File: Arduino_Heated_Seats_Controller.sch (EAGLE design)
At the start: 13 parts, among them U1 ULN2003AN, U2 M54564P

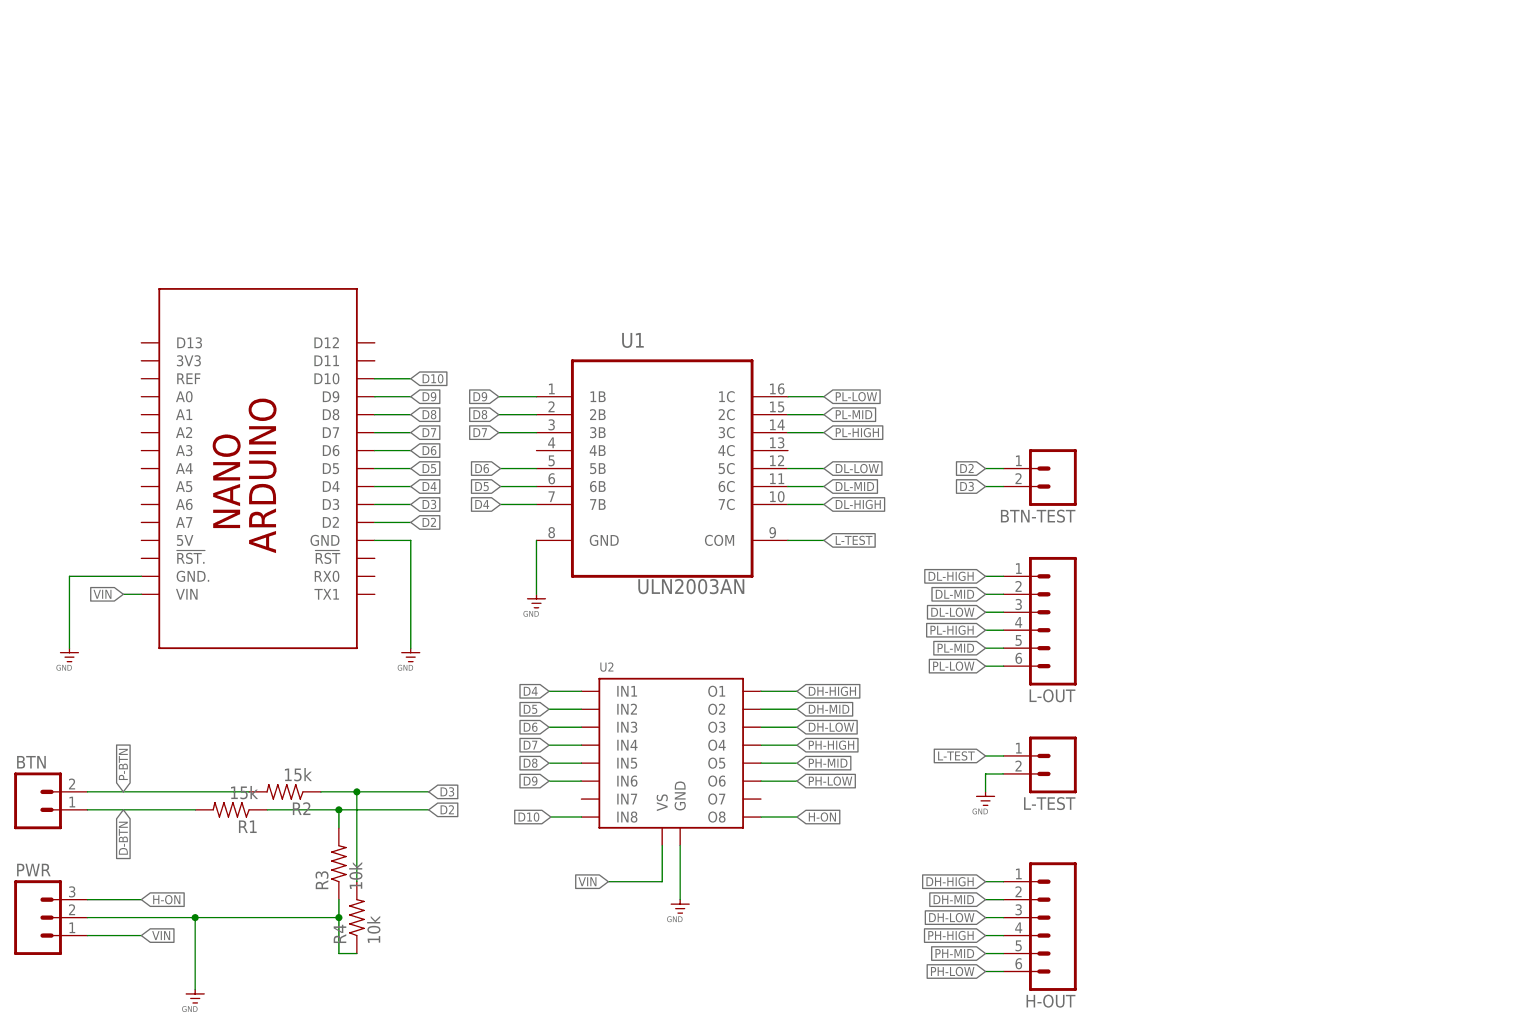
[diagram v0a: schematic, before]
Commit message: Initial work on rev3 underway (time for some sleep).
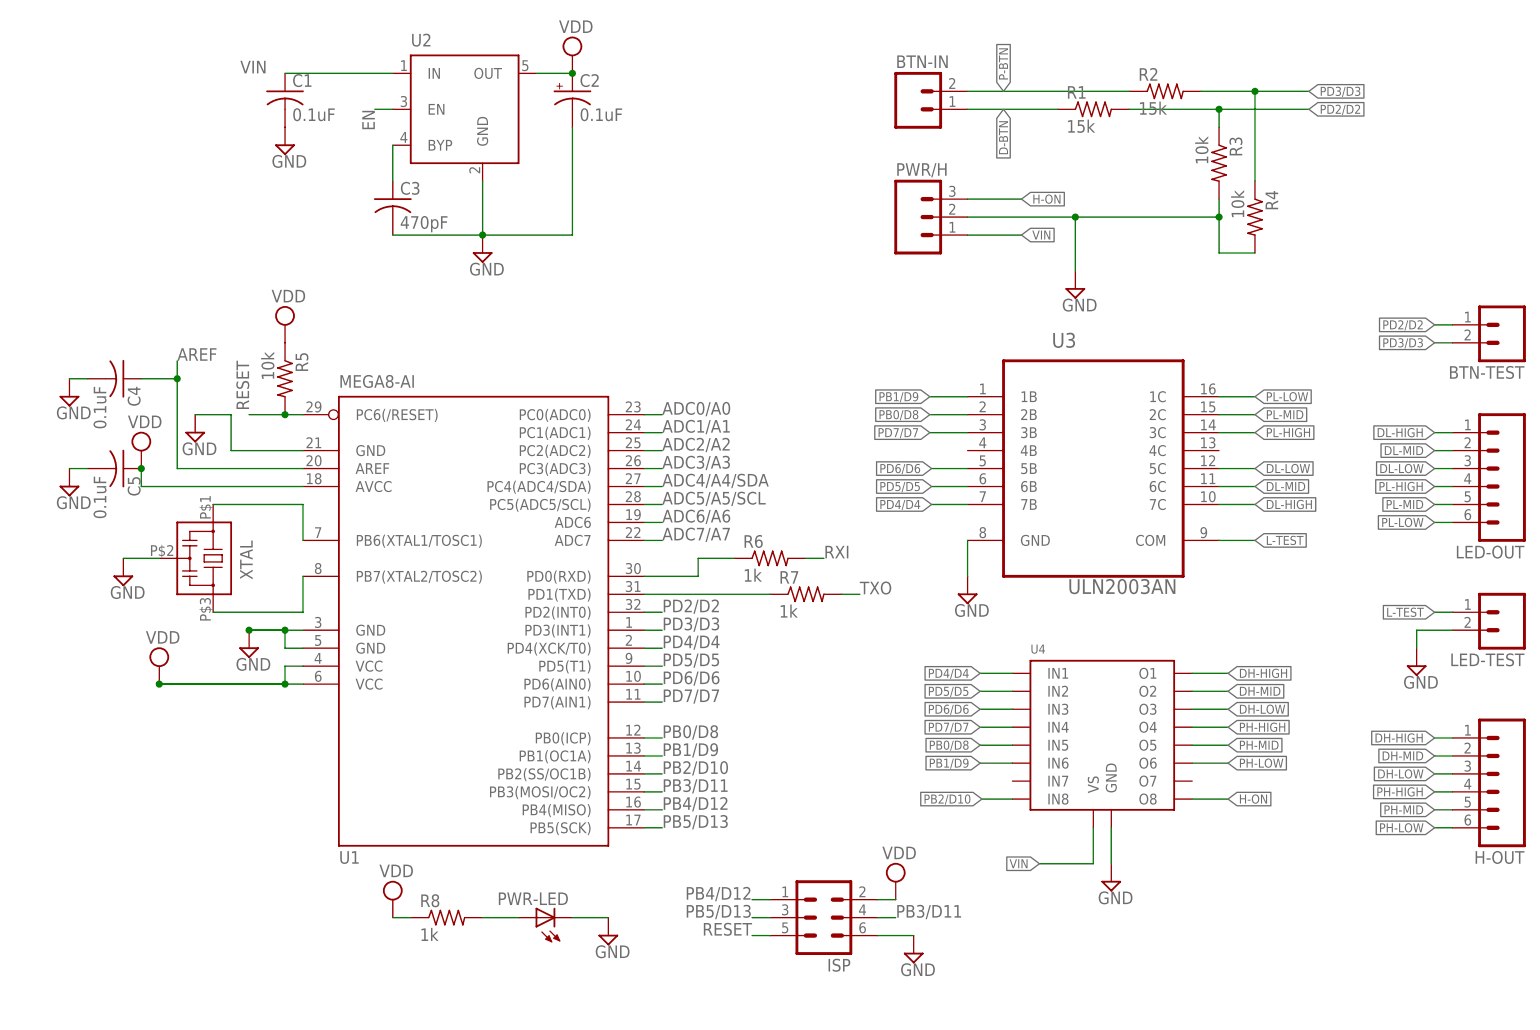
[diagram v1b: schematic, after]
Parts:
- removed BTN, L-TEST: M02PTH, SparkFun-Connectors:M02PTH
- removed L-OUT: (no value), SparkFun-Connectors:M06SIP
- removed PCB1: ARDUINO_NANO, E14_Arduino:ARDUINO_NANO
- removed PWR: (no value), SparkFun-Connectors:M03PTH
- added BTN-IN, LED-TEST: M02PTH, SparkFun-Connectors:M02PTH
- added C1, C4, C5: 0.1uF, rcl:C-USC0603
- added C2: 0.1uF, rcl:CPOL-USCT3216
- added C3: 470pF, rcl:C-USC0603
- added ISP: (no value), con-lstb:MA03-2
- added LED-OUT: (no value), SparkFun-Connectors:M06SIP
- added PWR-LED: (no value), led:LEDCHIP-LED0603
- added PWR/H: (no value), SparkFun-Connectors:M03PTH
- added R5: 10k, resistor:R-US_R0603
- added R6, R7, R8: 1k, resistor:R-US_R0603
- added U3: ULN2003AN, Texas Instruments_By_element14_Batch_1:ULN2003ANE4
- added U4: M54564FP, M54564P-FP:M54564FP
- added XTAL: CSTCE_V, murata-filter:CSTCE_V
- R1, R2, R3, R4: device SparkFun-Resistors:RESISTOR0603-RES -> resistor:R-US_R0603
- U1: value ULN2003AN -> MEGA8-AI; device Texas Instruments_By_element14_Batch_1:ULN2003ANE4 -> atmel:MEGA8-AI
- U2: value M54564P -> (none); device M54564P-FP:M54564P -> v-reg-micrel:MIC5219XX
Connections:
- removed net D10: PCB1.D10, U2.IN8
- removed net D2: BTN-TEST.1, PCB1.D2, R1.1, R3.2
- removed net D3: BTN-TEST.2, PCB1.D3, R2.1, R4.2
- removed net D4: PCB1.D4, U1.7B, U2.IN1
- removed net D5: PCB1.D5, U1.6B, U2.IN2
- removed net D6: PCB1.D6, U1.5B, U2.IN3
- removed net D7: PCB1.D7, U1.3B, U2.IN4
- removed net D8: PCB1.D8, U1.2B, U2.IN5
- removed net D9: PCB1.D9, U1.1B, U2.IN6
- new net ADC0/A0: U1.PC0(ADC0)
- new net ADC1/A1: U1.PC1(ADC1)
- new net ADC2/A2: U1.PC2(ADC2)
- new net ADC3/A3: U1.PC3(ADC3)
- new net ADC4/A4/SDA: U1.PC4(ADC4/SDA)
- new net ADC5/A5/SCL: U1.PC5(ADC5/SCL)
- new net ADC6/A6: U1.ADC6
- new net ADC7/A7: U1.ADC7
- new net AREF: C4.1, U1.AREF
- new net EN: U2.EN
- new net N$3: PWR-LED.A, R8.2
- new net N$4: C3.1, U2.BYP
- new net N$8: R6.1, U1.PD0(RXD)
- new net N$9: R7.1, U1.PD1(TXD)
- new net PB0/D8: U1.PB0(ICP), U3.2B, U4.IN5
- new net PB1/D9: U1.PB1(OC1A), U3.1B, U4.IN6
- new net PB2/D10: U1.PB2(SS/OC1B), U4.IN8
- new net PB3/D11: ISP.4, U1.PB3(MOSI/OC2)
- new net PB4/D12: ISP.1, U1.PB4(MISO)
- new net PB5/D13: ISP.3, U1.PB5(SCK)
- new net PB6: U1.PB6(XTAL1/TOSC1), XTAL.1
- new net PB7: U1.PB7(XTAL2/TOSC2), XTAL.3
- new net PD2/D2: BTN-TEST.1, R1.2, R3.1, U1.PD2(INT0)
- new net PD3/D3: BTN-TEST.2, R2.2, R4.1, U1.PD3(INT1)
- new net PD4/D4: U1.PD4(XCK/T0), U3.7B, U4.IN1
- new net PD5/D5: U1.PD5(T1), U3.6B, U4.IN2
- new net PD6/D6: U1.PD6(AIN0), U3.5B, U4.IN3
- new net PD7/D7: U1.PD7(AIN1), U3.3B, U4.IN4
- new net RESET: ISP.5, R5.2, U1.PC6(/RESET)
- new net RXI: R6.2
- new net TXO: R7.2
- new net VDD: C2.+, C5.1, ISP.2, R5.1, R8.1, U1.AVCC, U1.VCC@1, U1.VCC@2, U2.OUT
- net D-BTN: now also BTN-IN.1, R1.1; no longer BTN.1, R1.2
- net DH-HIGH: now also U4.O1; no longer U2.O1
- net DH-LOW: now also U4.O3; no longer U2.O3
- net DH-MID: now also U4.O2; no longer U2.O2
- net DL-HIGH: now also LED-OUT.1, U3.7C; no longer L-OUT.1, U1.7C
- net DL-LOW: now also LED-OUT.3, U3.5C; no longer L-OUT.3, U1.5C
- net DL-MID: now also LED-OUT.2, U3.6C; no longer L-OUT.2, U1.6C
- net GND: now also C1.2, C2.-, C3.2, C4.2, C5.2, ISP.6, LED-TEST.2, PWR-LED.C, PWR/H.2, R3.2, R4.2, U1.GND@1, U1.GND@2, U3.GND, U4.GND, XTAL.2; no longer L-TEST.2, PCB1.GND, PCB1.GND., PWR.2, R3.1, R4.1
- net H-ON: now also PWR/H.3, U4.O8; no longer PWR.3, U2.O8
- net L-TEST: now also LED-TEST.1, U3.COM; no longer L-TEST.1, U1.COM
- net P-BTN: now also BTN-IN.2, R2.1; no longer BTN.2, R2.2
- net PH-HIGH: now also U4.O4; no longer U2.O4
- net PH-LOW: now also U4.O6; no longer U2.O6
- net PH-MID: now also U4.O5; no longer U2.O5
- net PL-HIGH: now also LED-OUT.4, U3.3C; no longer L-OUT.4, U1.3C
- net PL-LOW: now also LED-OUT.6, U3.1C; no longer L-OUT.6, U1.1C
- net PL-MID: now also LED-OUT.5, U3.2C; no longer L-OUT.5, U1.2C
- net VIN: now also C1.1, PWR/H.1, U2.IN, U4.VS; no longer PCB1.VIN, PWR.1, U2.VS
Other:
- moved on the sheet: BTN-TEST, H-OUT, R1, R2, R3, R4
